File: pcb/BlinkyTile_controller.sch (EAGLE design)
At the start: 9 parts

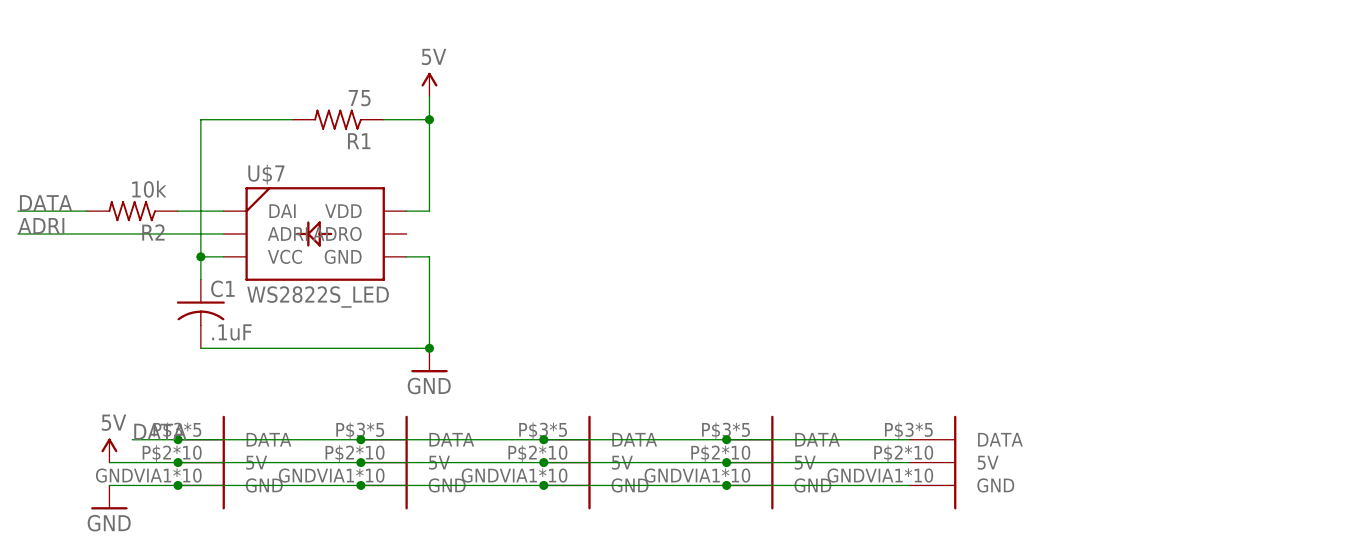
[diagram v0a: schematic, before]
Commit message: Rev E of pcb, control pcb
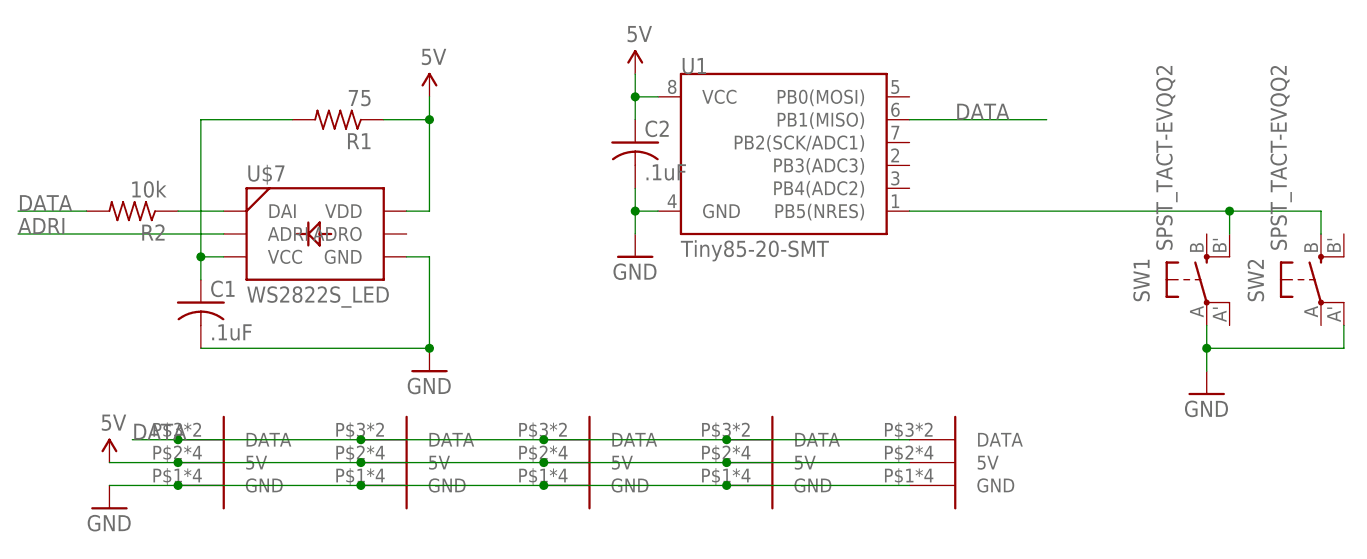
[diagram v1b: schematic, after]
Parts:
- added C2: .1uF, adafruit:C-USC0603
- added SW1, SW2: SPST_TACT-EVQQ2, adafruit:SPST_TACT-EVQQ2
- added U1: Tiny85-20-SMT, SparkFun-DigitalIC:ATTINY45TINY85-20-SMT
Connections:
- new net N$3: SW1.S1, SW2.S, U1.PB5(NRES)
- net 5V: now also C2.1, U1.VCC
- net DATA: now also U1.PB1(MISO)
- net GND: now also C2.2, SW1.P, SW2.P1, U1.GND
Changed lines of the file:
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@@
 <part name="U$6" library="dodocohedreled" deviceset="D_EDGE" device="SLOT"/>
 <part name="U$7" library="blinkinlabs" deviceset="WS2822S_LED" device=""/>
+<part name="U1" library="SparkFun-DigitalIC" deviceset="ATTINY45" device="TINY85-20-SMT" value="Tiny85-20-SMT"/>
+<part name="SUPPLY1" library="SparkFun-Aesthetics" deviceset="5V" device=""/>
+<part name="GND3" library="SparkFun-Aesthetics" deviceset="GND" device=""/>
+<part name="C2" library="adafruit" deviceset="C-US" device="C0603" value=".1uF"/>
+<part name="SW1" library="adafruit" deviceset="SPST_TACT" device="-EVQQ2"/>
+<part name="SW2" library="adafruit" deviceset="SPST_TACT" device="-EVQQ2"/>
+<part name="GND4" library="SparkFun-Aesthetics" deviceset="GND" device=""/>
 </parts>
 <sheets>
@@
 <instance part="U$6" gate="G$1" x="104.14" y="58.42"/>
 <instance part="U$7" gate="G$1" x="58.42" y="81.28"/>
+<instance part="U1" gate="G$1" x="111.76" y="88.9"/>
+<instance part="SUPPLY1" gate="G$1" x="93.98" y="99.06"/>
+<instance part="GND3" gate="1" x="93.98" y="78.74"/>
+<instance part="C2" gate="G$1" x="93.98" y="91.44"/>
+<instance part="SW1" gate="G$1" x="157.48" y="76.2"/>
+<instance part="SW2" gate="G$1" x="170.18" y="76.2"/>
+<instance part="GND4" gate="1" x="157.48" y="63.5"/>
 </instances>
 <busses>
@@
 <junction x="71.12" y="93.98"/>
 </segment>
+<segment>
+<pinref part="U1" gate="G$1" pin="VCC"/>
+<pinref part="SUPPLY1" gate="G$1" pin="5V"/>
+<wire x1="96.52" y1="96.52" x2="93.98" y2="96.52" width="0.1524" layer="91"/>
+<wire x1="93.98" y1="96.52" x2="93.98" y2="99.06" width="0.1524" layer="91"/>
+<pinref part="C2" gate="G$1" pin="1"/>
+<wire x1="93.98" y1="96.52" x2="93.98" y2="93.98" width="0.1524" layer="91"/>
+<junction x="93.98" y="96.52"/>
+</segment>
 </net>
 <net name="GND" class="0">
@@
 <pinref part="U$6" gate="G$1" pin="GND"/>
 <junction x="104.14" y="53.34"/>
+</segment>
+<segment>
+<pinref part="U1" gate="G$1" pin="GND"/>
+<pinref part="GND3" gate="1" pin="GND"/>
+<wire x1="96.52" y1="83.82" x2="93.98" y2="83.82" width="0.1524" layer="91"/>
+<wire x1="93.98" y1="83.82" x2="93.98" y2="81.28" width="0.1524" layer="91"/>
+<pinref part="C2" gate="G$1" pin="2"/>
+<wire x1="93.98" y1="86.36" x2="93.98" y2="83.82" width="0.1524" layer="91"/>
+<junction x="93.98" y="83.82"/>
+</segment>
+<segment>
+<wire x1="172.72" y1="68.58" x2="157.48" y2="68.58" width="0.1524" layer="91"/>
+<pinref part="SW1" gate="G$1" pin="P"/>
+<wire x1="157.48" y1="71.12" x2="157.48" y2="68.58" width="0.1524" layer="91"/>
+<pinref part="GND4" gate="1" pin="GND"/>
+<junction x="157.48" y="68.58"/>
+<wire x1="157.48" y1="68.58" x2="157.48" y2="66.04" width="0.1524" layer="91"/>
+<pinref part="SW2" gate="G$1" pin="P1"/>
+<wire x1="172.72" y1="71.12" x2="172.72" y2="68.58" width="0.1524" layer="91"/>
 </segment>
 </net>
@@
 <junction x="104.14" y="58.42"/>
 </segment>
+<segment>
+<pinref part="U1" gate="G$1" pin="PB1(MISO)"/>
+<wire x1="124.46" y1="93.98" x2="139.7" y2="93.98" width="0.1524" layer="91"/>
+<label x="129.54" y="93.98" size="1.778" layer="95"/>
+</segment>
 </net>
 <net name="N$1" class="0">
@@
 </segment>
 </net>
+<net name="N$3" class="0">
+<segment>
+<pinref part="U1" gate="G$1" pin="PB5(NRES)"/>
+<wire x1="124.46" y1="83.82" x2="160.02" y2="83.82" width="0.1524" layer="91"/>
+<pinref part="SW2" gate="G$1" pin="S"/>
+<wire x1="160.02" y1="83.82" x2="170.18" y2="83.82" width="0.1524" layer="91"/>
+<wire x1="170.18" y1="83.82" x2="170.18" y2="81.28" width="0.1524" layer="91"/>
+<pinref part="SW1" gate="G$1" pin="S1"/>
+<wire x1="160.02" y1="81.28" x2="160.02" y2="83.82" width="0.1524" layer="91"/>
+<junction x="160.02" y="83.82"/>
+</segment>
+</net>
